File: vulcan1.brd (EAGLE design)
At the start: 101.6 x 100 mm, 45 parts, among them U1 SD_CARD_SOCKET4UCON

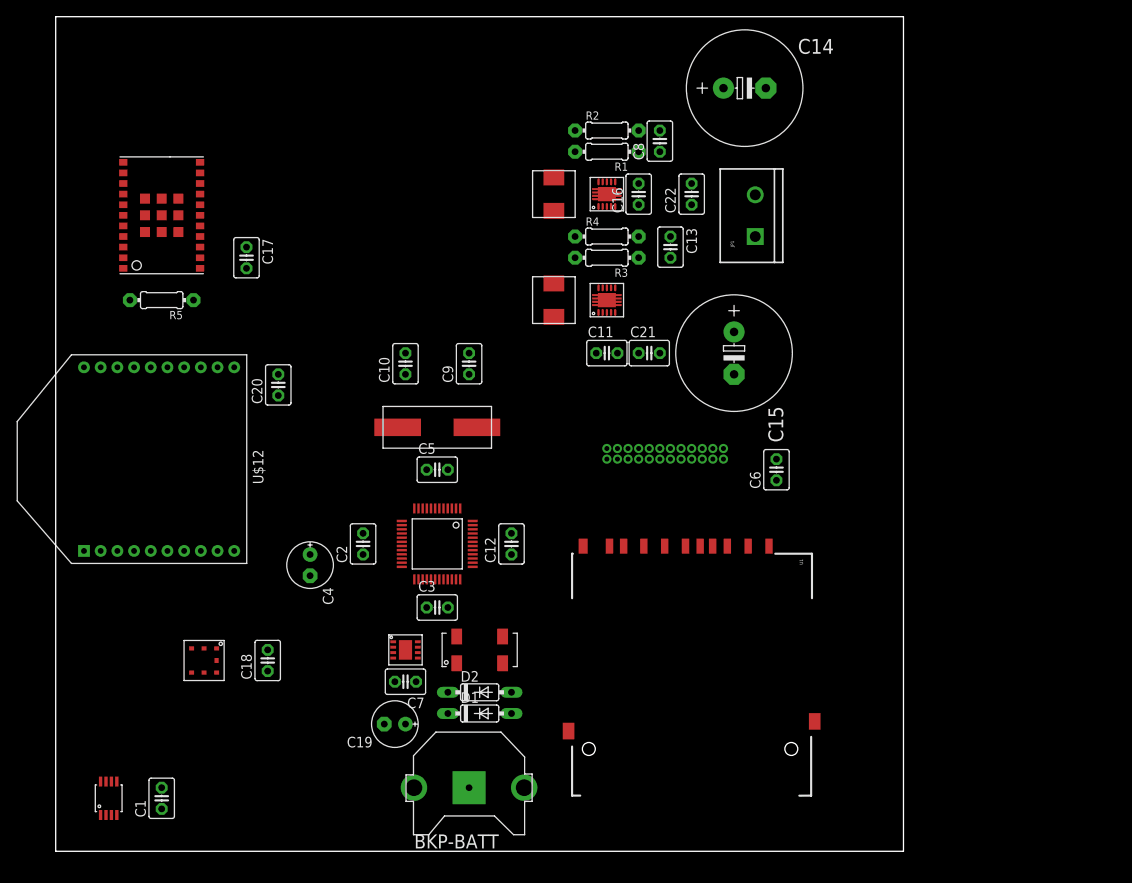
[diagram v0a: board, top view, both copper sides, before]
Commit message: update-all but RF traces and gnd plane done
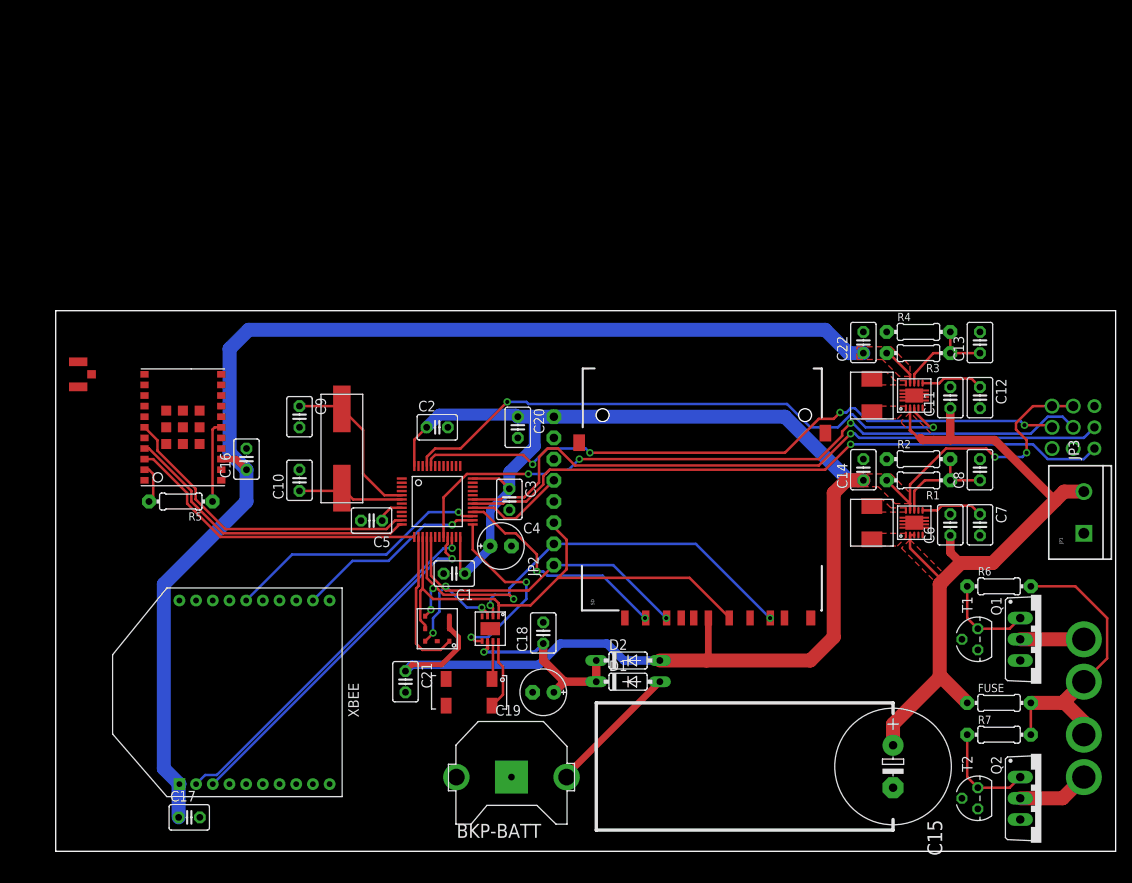
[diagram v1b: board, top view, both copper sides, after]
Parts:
- removed U$11: BMP183, vulcan-1:LGA-7
- removed U$12: XBEE, adafruit:XBEE
- removed U$13: 2X24HEADER, vulcan-1:1.27MM2X12
- removed U$8: DS1347, vulcan-1:TDFN-T822-2
- removed U1: SD_CARD_SOCKET4UCON, SparkFun-Connectors:SDCARD_4UCONN
- added A2200-A: A2200-A, vulcan-1:GPS-MODULE
- added BMP183: BMP183, vulcan-1:LGA-7
- added DS1347: DS1347, vulcan-1:TDFN-T822-2
- added FUSE: FUSE, adafruit:0204/7
- added JP2: (no value), adafruit:1X08-CLEANBIG
- added JP3: (no value), adafruit:1X03-CLEANBIG
- added Q1, Q2: IRF540, transistor-power:TO220BV
- added R6, R7: 10k, adafruit:0204/7
- added SD: SD_CARD_SOCKET4UCON, SparkFun-Connectors:SDCARD_4UCONN
- added T1, T2: 2N3904, transistor:TO92
- added TPS63060-A, TPS63060-B: TPS63060, vulcan-1:PWSON-N10
- added XBEE: XBEE, adafruit:XBEE
- C14: value 4700uf -> .1u; device adafruit:E5-13 -> adafruit:C025-030X050
- U$2: value A2200-A -> 2X3; device vulcan-1:GPS-MODULE -> vulcan-1:2X3
- U$3, U$4: value TPS63060 -> 1X2BIG; device vulcan-1:PWSON-N10 -> vulcan-1:1X2BIG
- U$7: value AD8494ARMZ -> SMA; device vulcan-1:MSOP-8 -> vulcan-1:SMA
- moved U$2 112.1 mm to (121.9, 50.8), turned to 270 degrees
- moved U$3 79.9 mm to (123.2, 22.9), turned to 90 degrees
- moved U$4 79.0 mm to (123.2, 11.4), turned to 270 degrees
- moved C7 71.4 mm to (110.7, 39.1), turned to 270 degrees
- moved C17 67.4 mm to (16.0, 4.06), turned to 0 degrees
- moved C12 58.8 mm to (110.7, 54.4), turned to 270 degrees
- moved C16 56.7 mm to (22.9, 47.0)
- moved C8 55.0 mm to (110.7, 45.7)
- moved U$6 54.8 mm to (97.8, 39.4)
- moved R2 54.3 mm to (103.4, 47.0)
- moved R1 54.3 mm to (103.4, 44.5)
- moved C15 53.1 mm to (100.3, 10.2)
- moved JP1 53.1 mm to (123.2, 38.1)
- moved U$7 50.9 mm to (2.79, 57.1), turned to 90 degrees
- moved C21 49.0 mm to (41.9, 20.3), turned to 270 degrees
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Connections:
- removed net N$23: U$2.6
- removed net N$24: U$7.1, U$7.8
- removed net N$30: U$7.5, U$7.6
- removed net SPI-NSS: U$1.14
- removed net VB-EN: U$4.3
- new net EMATCH1: T1.2
- new net EMATCH2: T2.2
- new net GPS-CS: A2200-A.6, U$1.11
- new net N$1: Q1.G, R6.1, T1.1
- new net N$13: Q1.D, U$3.2
- new net N$16: Q2.G, R7.1, T2.1
- new net N$17: Q2.D, U$4.2
- new net VB-CS: TPS63060-B.3, U$1.45
- new net VBAT-F: FUSE.2, R6.2, R7.2, U$3.1, U$4.1
- net 3.3A: now also BMP183.2, BMP183.3, C14.1, JP2.8, SD.4, TPS63060-A.9, U$2.1, U$2.2; no longer C22.1, U$11.2, U$11.3, U$13.10, U$13.11, U$13.12, U$3.9, U$7.7, U1.4
- net 3.3B: now also A2200-A.20, C22.1, TPS63060-B.9, XBEE.1; no longer U$12.1, U$2.20, U$4.9
- net ACC-CS: now also JP2.5, U$1.29; no longer U$13.6
- net ACC-FLAG: now also JP2.6; no longer U$13.7
- net ACC-RST: now also JP2.4; no longer U$13.8
- net BOOT0: now also U$2.3
- net BOOT1: now also U$2.4
- net GND: now also A2200-A.10, A2200-A.7, A2200-A.8, A2200-A.P$1, A2200-A.P$2, A2200-A.P$3, A2200-A.P$4, A2200-A.P$5, A2200-A.P$6, A2200-A.P$7, A2200-A.P$8, A2200-A.P$9, BMP183.7, C14.2, DS1347.4, JP2.7, JP3.3, Q1.S, Q2.S, SD.3, SD.6, T1.3, T2.3, TPS63060-A.4, TPS63060-A.5, TPS63060-A.7, TPS63060-A.PGND_1, TPS63060-A.PGND_2, TPS63060-A.PGND_3, TPS63060-A.PGND_4, TPS63060-A.PGND_5, TPS63060-A.PGND_6, TPS63060-A.PGND_7, TPS63060-A.PGND_8, TPS63060-A.PGND_9, TPS63060-B.4, TPS63060-B.5, TPS63060-B.7, TPS63060-B.PGND_1, TPS63060-B.PGND_2, TPS63060-B.PGND_3, TPS63060-B.PGND_4, TPS63060-B.PGND_5, TPS63060-B.PGND_6, TPS63060-B.PGND_7, TPS63060-B.PGND_8, TPS63060-B.PGND_9, U$2.5, U$2.6, XBEE.10; no longer U$11.7, U$12.10, U$13.13, U$13.14, U$13.15, U$2.10, U$2.7, U$2.8, U$2.P$1, U$2.P$2, U$2.P$3, U$2.P$4, U$2.P$5, U$2.P$6, U$2.P$7, U$2.P$8, U$2.P$9, U$3.4, U$3.5, U$3.7, U$3.PGND_1, U$3.PGND_2, U$3.PGND_3, U$3.PGND_4, U$3.PGND_5, U$3.PGND_6, U$3.PGND_7, U$3.PGND_8, U$3.PGND_9, U$4.4, U$4.5, U$4.7, U$4.PGND_1, U$4.PGND_2, U$4.PGND_3, U$4.PGND_4, U$4.PGND_5, U$4.PGND_6, U$4.PGND_7, U$4.PGND_8, U$4.PGND_9, U$7.2, U$7.3, U$8.4, U1.3, U1.6
- net GPS-ANT: now also A2200-A.11, U$7.3; no longer U$2.11
- net N$11: now also TPS63060-A.6; no longer U$3.6
- net N$12: now also DS1347.6; no longer U$8.6
- net N$14: now also TPS63060-A.8; no longer U$3.8
- net N$15: now also TPS63060-B.8; no longer U$4.8
- net N$18: now also TPS63060-B.6; no longer U$4.6
- net N$20: now also A2200-A.2; no longer U$2.2
- net N$21: now also A2200-A.17; no longer U$2.17
- net N$3: now also TPS63060-B.1; no longer U$4.1
- net N$4: now also TPS63060-B.10; no longer U$4.10
- net N$5: now also TPS63060-A.1; no longer U$3.1
- net N$6: now also TPS63060-A.10; no longer U$3.10
- net N$7: now also DS1347.7; no longer U$8.7
- net N$8: now also DS1347.8; no longer U$8.8
- net PS-CS: now also BMP183.1, U$1.14; no longer U$11.1
- net RTC-CS: now also DS1347.5, U$1.25; no longer U$8.5
- net SD-CS: now also SD.1, U$1.28; no longer U1.1
- net SPI-MISO: now also BMP183.4, DS1347.2, JP2.2, SD.7; no longer U$11.4, U$13.4, U$8.2, U1.7
- net SPI-MOSI: now also BMP183.6, DS1347.3, JP2.1, SD.2; no longer U$11.6, U$13.5, U$8.3, U1.2
- net SPI-SCK: now also BMP183.5, DS1347.1, JP2.3, SD.5; no longer U$11.5, U$13.3, U$8.1, U1.5
- net USART1-RX: now also JP3.2
- net USART1-TX: now also JP3.1
- net USART2-RX: now also A2200-A.3; no longer U$2.3
- net USART2-TX: now also A2200-A.4; no longer U$1.21, U$2.4
- net USART3-CTS: now also XBEE.12; no longer U$12.12
- net USART3-RTS: now also XBEE.16; no longer U$12.16
- net USART3-RX: now also XBEE.2; no longer U$12.2
- net USART3-TX: now also U$1.21, XBEE.3; no longer U$12.3
- net VBAT: now also FUSE.1, TPS63060-A.2, TPS63060-A.3, TPS63060-B.2; no longer C14.+, U$3.2, U$3.3, U$4.2
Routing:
- net 3.3A: track 0.00 -> 221.7 mm, vias 0 -> 2
- net 3.3B: track 0.00 -> 148.4 mm
- net VBAT: track 0.00 -> 90.9 mm
- net BOOT1: track 0.00 -> 86.1 mm, vias 0 -> 3
- net USART1-RX: track 0.00 -> 82.0 mm, vias 0 -> 1
- net BOOT0: track 0.00 -> 80.2 mm, vias 0 -> 4
- net USART1-TX: track 0.00 -> 79.3 mm, vias 0 -> 1
- net VB-CS: track 0.00 -> 70.5 mm, vias 0 -> 2
- net SPI-MISO: track 0.00 -> 63.8 mm, vias 0 -> 5
- net SPI-SCK: track 0.00 -> 61.5 mm
- net SPI-MOSI: track 0.00 -> 52.2 mm, vias 0 -> 4
- net USART3-RX: track 0.00 -> 43.7 mm, vias 0 -> 1
- net USART3-TX: track 0.00 -> 42.9 mm, vias 0 -> 1
- net GPS-CS: track 0.00 -> 37.8 mm
- net USART2-RX: track 0.00 -> 36.9 mm
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- added copper zone on layer 1, net 3.3A
- added copper zone on layer 1, net 3.3B
- added copper zone on layer 1, net N$3
- added copper zone on layer 1, net N$4
- added copper zone on layer 1, net N$5
- added copper zone on layer 1, net N$6
- added copper zone on layer 1, net VBAT
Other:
- board size 101.6 x 100 mm -> 127 x 64.8 mm
